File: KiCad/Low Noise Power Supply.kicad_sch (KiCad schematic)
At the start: 27 parts, among them Q401 FMMT614TA, Q402 FMMT734, U401 L78L15_SOT89, U402 PESE1-S5-S24-M, U403 L78L05, U404 L79L15_SOT89

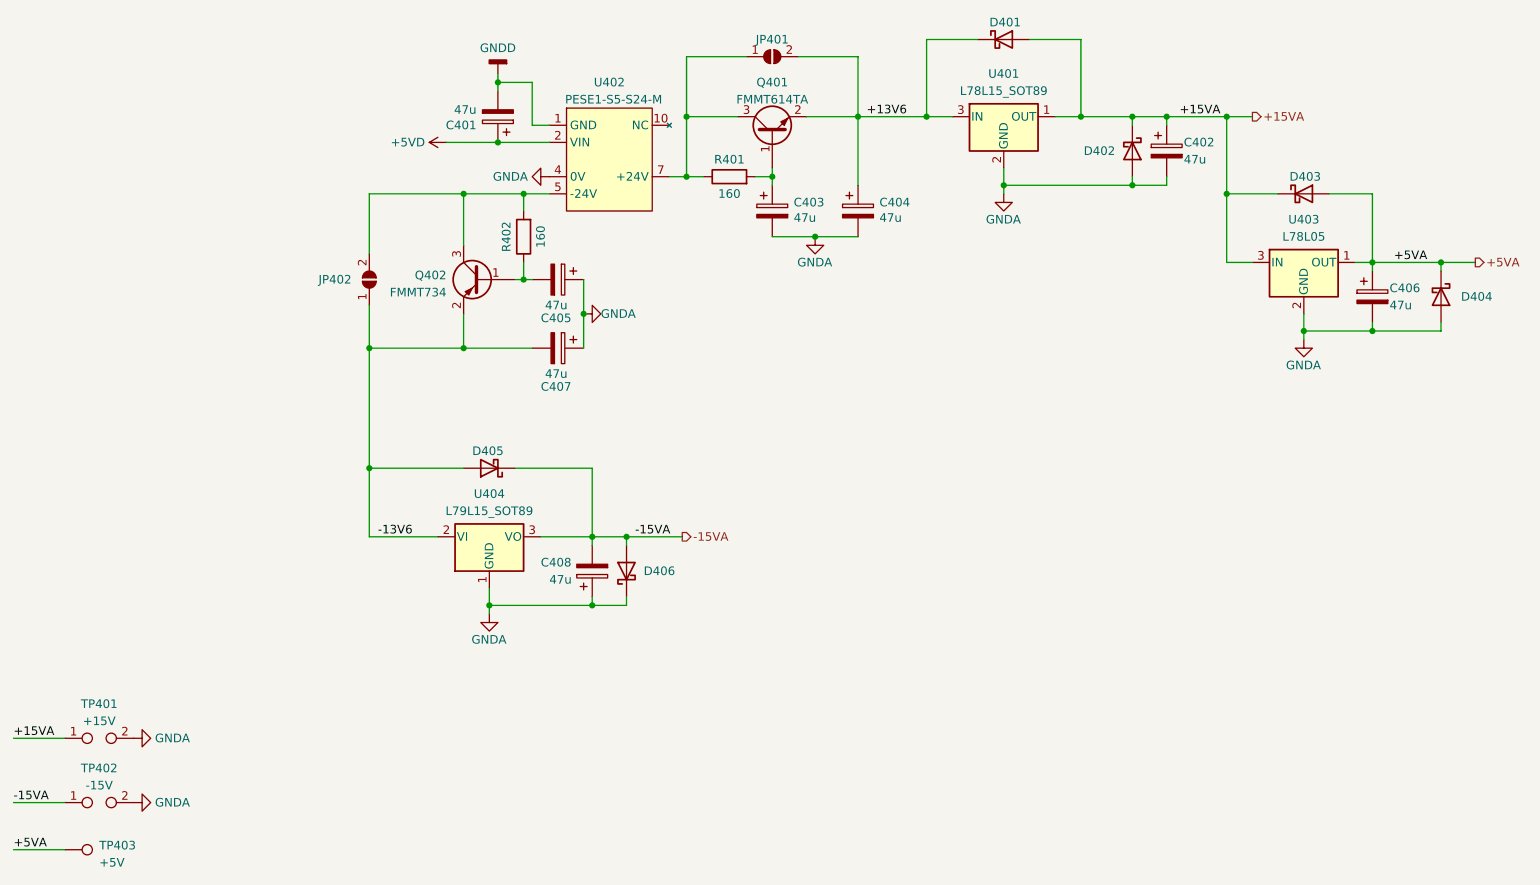
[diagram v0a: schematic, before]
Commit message: Cleaned up a few things
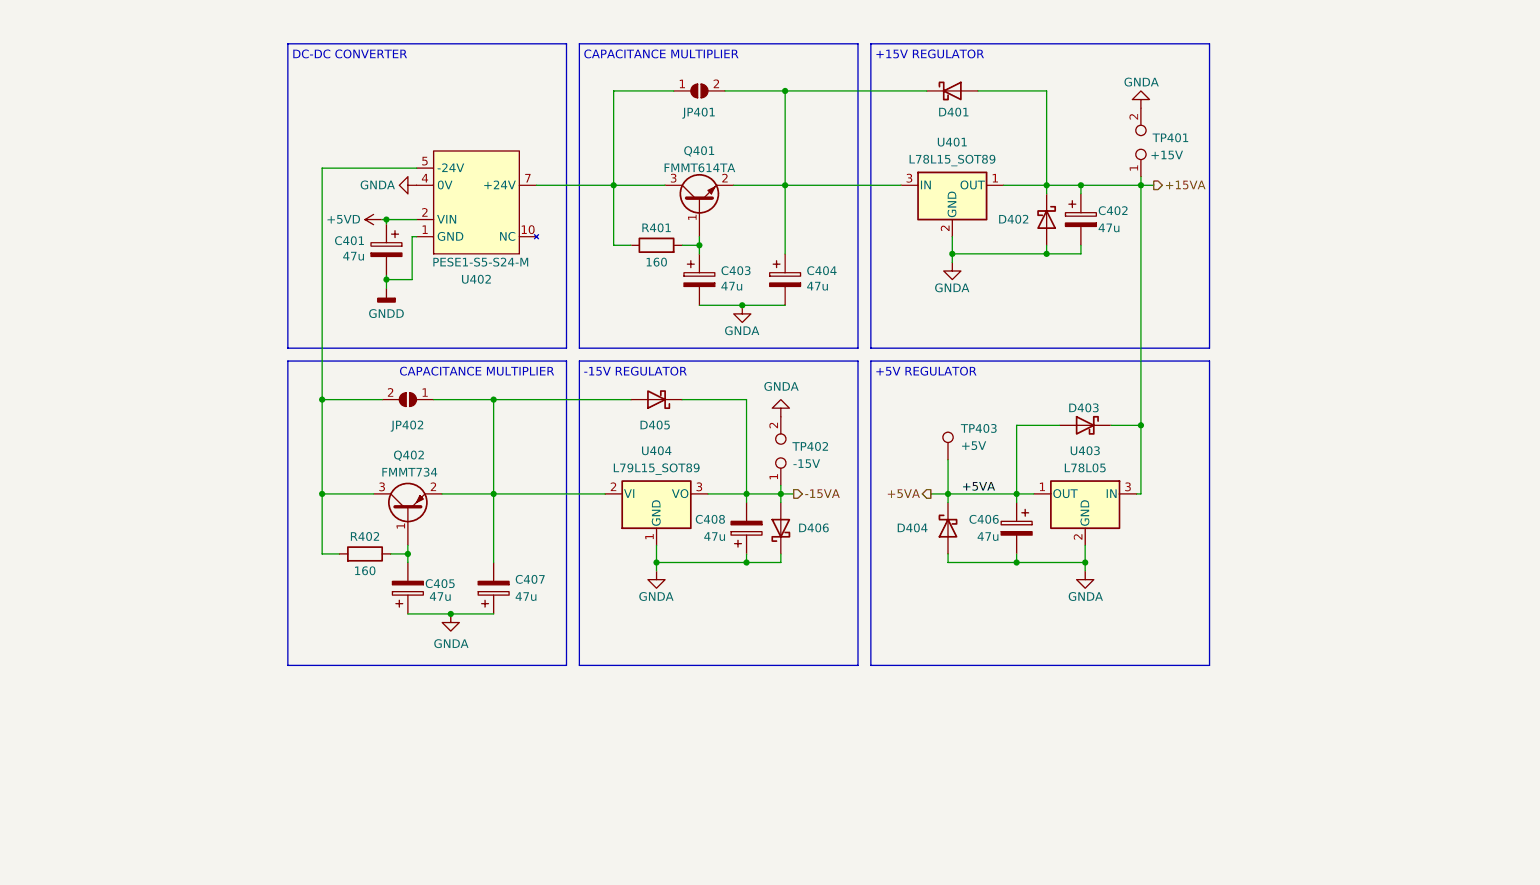
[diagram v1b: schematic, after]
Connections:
- net +13V6: no longer names the net of C404.1, D401.1 (K), JP401.2 (B), Q401.2 (E), U401.3 (IN)
- net -13V6: no longer names the net of C407.2, D405.2 (A), JP402.1 (A), Q402.2 (E), U404.2 (VI)
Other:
- note added: "+15V REGULATOR"
- note added: "+5V REGULATOR"
- note added: "-15V REGULATOR"
- note added: "CAPACITANCE MULTIPLIER"
- note added: "DC-DC CONVERTER"
- company: (none) -> M Morano
- moved on the sheet: C401, C402, C403, C404, C405, C406, C407, C408, D401, D402, D403, D404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
